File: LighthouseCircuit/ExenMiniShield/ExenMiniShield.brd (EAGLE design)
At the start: 25.4 x 16.5 mm, 31 parts, among them J3 SM02B-SRSS

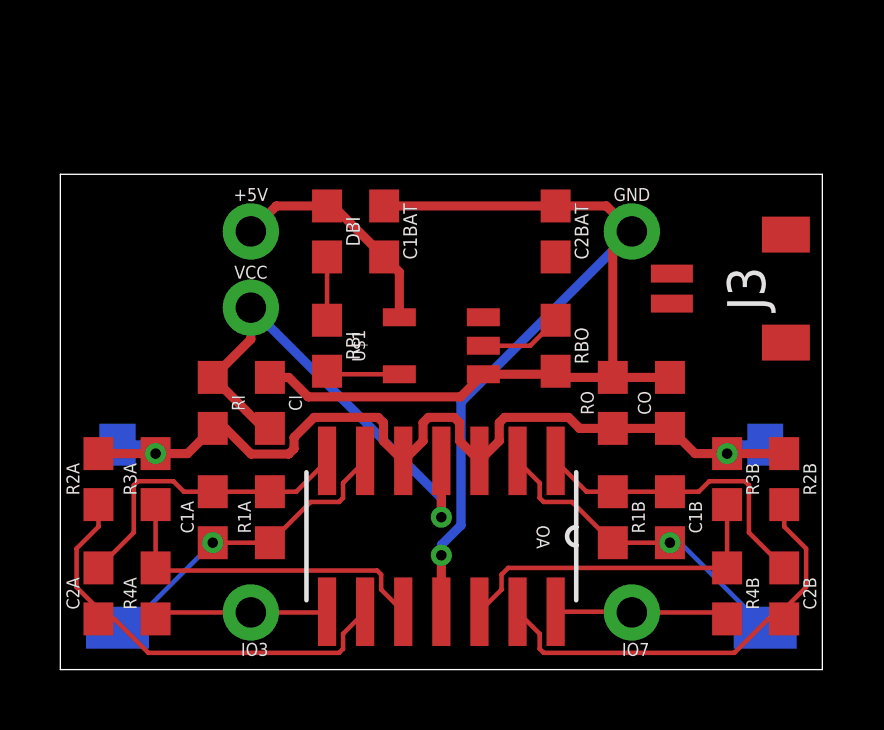
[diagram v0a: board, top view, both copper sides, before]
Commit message: Reached a point where auto-drive mode is consistent and reliable.
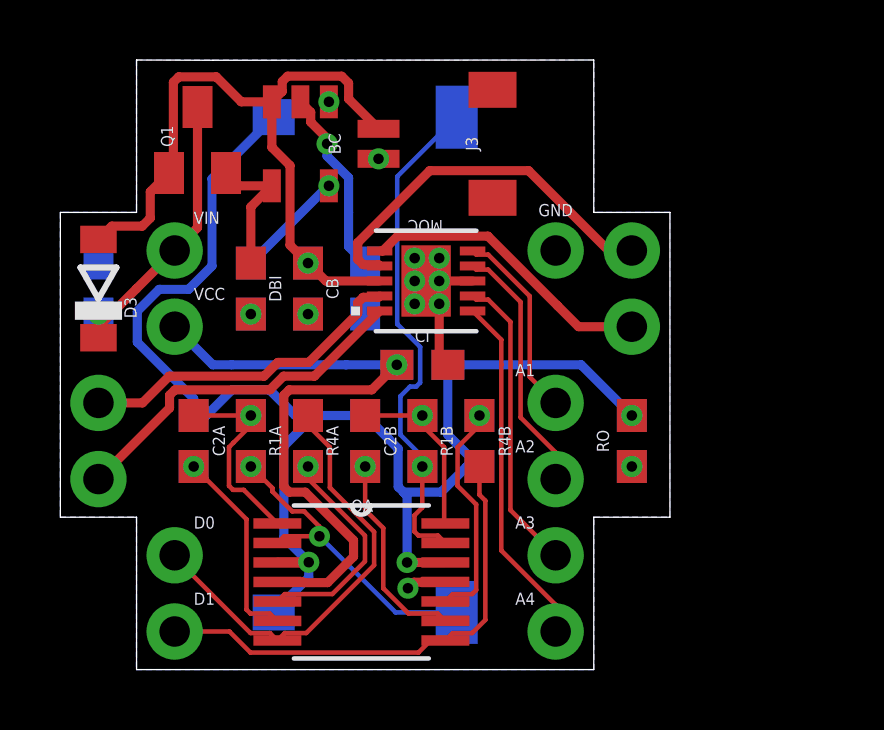
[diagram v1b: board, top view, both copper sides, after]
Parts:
- removed +5V, IO3, IO7: (no value), SparkFun-Connectors:1X01_NO_SILK
- removed C1BAT: 10uF, ZippyComponentLibrary:PASSIVE-0603
- removed C2BAT: 4.7uF, ZippyComponentLibrary:PASSIVE-0603
- removed D2: PHOTODIODEBPW, ZippyComponentLibrary:BPW34_BP104_SMD
- removed U$1: BATTERYCHARGER, ZippyComponentLibrary:SOT-753
- added A1, A2, A3, A4, D0, MA01, MA02, MB01, MBO2, VIN: (no value), SparkFun-Connectors:1X01_NO_SILK
- added BC: BATTERYCHARGER, ZippyComponentLibrary:SOT-753
- added C1: 10uF, ZippyComponentLibrary:PASSIVE-0603
- added C2: 4.7uF, ZippyComponentLibrary:PASSIVE-0603
- added CB: 10μF, SparkFun-Capacitors:0603
- added D3: MBR120, tinycircuits:SOD-123FL
- added DI0, DI1: PHOTODIODEBPW, ZippyComponentLibrary:BPW34_BP104_SMD
- added MOC: A3901SEJTR-T, ZippyComponentLibrary:DFN-10_DD
- added Q1: DMP2035U, tinycircuits:SOT23
- D1: value PHOTODIODEBPW -> (none); device ZippyComponentLibrary:BPW34_BP104_SMD -> SparkFun-Connectors:1X01_NO_SILK
- GND: value SINGLE-THROUGH-HOLE -> (none); device ZippyComponentLibrary:SINGLE-THROUGH-HOLE -> SparkFun-Connectors:1X01_NO_SILK
- J3: value SM02B-SRSS -> BATTERY
- OA: value TLV2464IDM -> TLV2464IPW; device ZippyComponentLibrary:D14-M -> ZippyComponentLibrary:PW14
- moved C2B 14.9 mm to (10.2, 7.62)
- moved R2B 14.0 mm to (10.2, 7.62), flipped to the bottom
- moved J3 10.9 mm to (13.1, 17.5)
- moved R4B 9.69 mm to (14.0, 7.62)
- moved C1B 8.64 mm to (12.1, 7.62), flipped to the bottom
- moved R3B 8.35 mm to (14.0, 7.62), flipped to the bottom, turned to 270 degrees
- moved R4A 7.18 mm to (8.26, 7.62), turned to 90 degrees
- moved RI 7.10 mm to (12.1, 10.2), flipped to the bottom, turned to 0 degrees
- moved R1B 6.84 mm to (12.1, 7.62)
- moved RBO 6.63 mm to (10.2, 12.7), flipped to the bottom
- moved C2A 5.99 mm to (4.45, 7.62)
- moved R3A 5.24 mm to (8.26, 7.62), flipped to the bottom
- moved CI 5.24 mm to (12.1, 10.2), turned to 0 degrees
- moved D1 3.70 mm to (3.81, 1.27), flipped to the top, turned to 0 degrees
- moved R2A 3.42 mm to (4.45, 7.62), flipped to the bottom
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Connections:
- removed net +5V: +5V.1, C1BAT.2, DBI.1, U$1.VDD
- removed net IO3: IO3.1, OA.8, R4A.2
- removed net IO7: IO7.1, OA.14, R4B.2
- new net D0: D0.1, OA.7, R4A.2
- new net D1: D1.1, OA.8, R4B.2
- new net MA01: MBO2.1, MOC.7
- new net MA02: MB01.1, MOC.6
- new net MB01: MA02.1, MOC.10
- new net MB02: MA01.1, MOC.9
- new net N$4: A1.1, MOC.5
- new net N$5: A2.1, MOC.4
- new net N$6: A4.1, MOC.1
- new net N$7: A3.1, MOC.2
- new net VDD: BC.VDD, DBI.1, Q1.E
- new net VIN: C1.2, D3.C, Q1.C, VIN.1
- net D1IN: now also DI1.CATHODE, OA.13; no longer D2.CATHODE, OA.2
- net D1OA2P: now also OA.9; no longer OA.13
- net D1OAOUT1: now also OA.14; no longer OA.1
- net D2IN: now also DI0.CATHODE, OA.2; no longer D1.CATHODE, OA.6
- net D2OA1OUT: now also OA.1; no longer OA.7
- net D2OA2N: now also OA.5; no longer OA.10
- net D2OA2P: now also OA.6; no longer OA.9
- net GND: now also BC.VSS, C1.1, C2.1, CB.1, MOC.11, MOC.3; no longer C1BAT.1, C2BAT.1, U$1.VSS
- net LVCC: now also DI0.ANODE, DI1.ANODE, OA.12; no longer D1.ANODE, D2.ANODE, OA.5
- net N$11: now also OA.10; no longer OA.12
- net N$2: now also BC.STAT; no longer U$1.STAT
- net N$3: now also BC.PROG; no longer U$1.PROG
- net VBAT: now also BC.VBAT, C2.2, CB.2, D3.A, MOC.8, Q1.B; no longer C2BAT.2, U$1.VBAT
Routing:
- net GND: track 43.1 -> 9.14 mm, vias 1 -> 11
- net VBAT: track 0.00 -> 24.2 mm, vias 0 -> 1
- net LVCC: track 31.4 -> 48.7 mm, vias 2 -> 3
- net D1: track 0.00 -> 16.3 mm
- net D0: track 0.00 -> 14.8 mm
- net MA01: track 0.00 -> 12.6 mm
- net MB01: track 0.00 -> 11.9 mm
- net N$6: track 0.00 -> 11.8 mm
- net MB02: track 0.00 -> 11.1 mm
- net N$7: track 0.00 -> 10.0 mm
- net MA02: track 0.00 -> 9.86 mm
- net VIN: track 0.00 -> 9.85 mm, vias 0 -> 1
- net N$5: track 0.00 -> 8.48 mm
- net D2OA2P: track 14.6 -> 6.68 mm, vias 0 -> 1
- net D1OA2P: track 14.6 -> 6.83 mm, vias 0 -> 1
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- added copper zone on layer 16, net GND
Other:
- board size 25.4 x 16.5 mm -> 20.3 x 20.3 mm
- board text removed: "Designed, Manufactured, and Assembled by Kyle Davis"
